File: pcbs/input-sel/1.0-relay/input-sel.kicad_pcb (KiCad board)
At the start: 2 copper layers, 85 x 55 mm, 54 parts, among them J1 Conn_01x03_Pin, J10 Conn_01x04_Pin, J2 Conn_01x03_Pin, J3 Conn_01x03_Pin, J4 Conn_01x03_Pin, J5 Conn_01x03_Pin, J6 Conn_01x03_Pin, J7 Conn_01x02_Pin, J8 Conn_01x02_Pin, J9 Conn_01x03_Pin, K1 EC2-5NU, K2 EC2-5NU, K3 EC2-5NU, K4 EC2-5NU, K5 EC2-5NU, K6 EC2-5NU, U1 CD74AC238, U2 TCMT4600, U3 TCMT4600

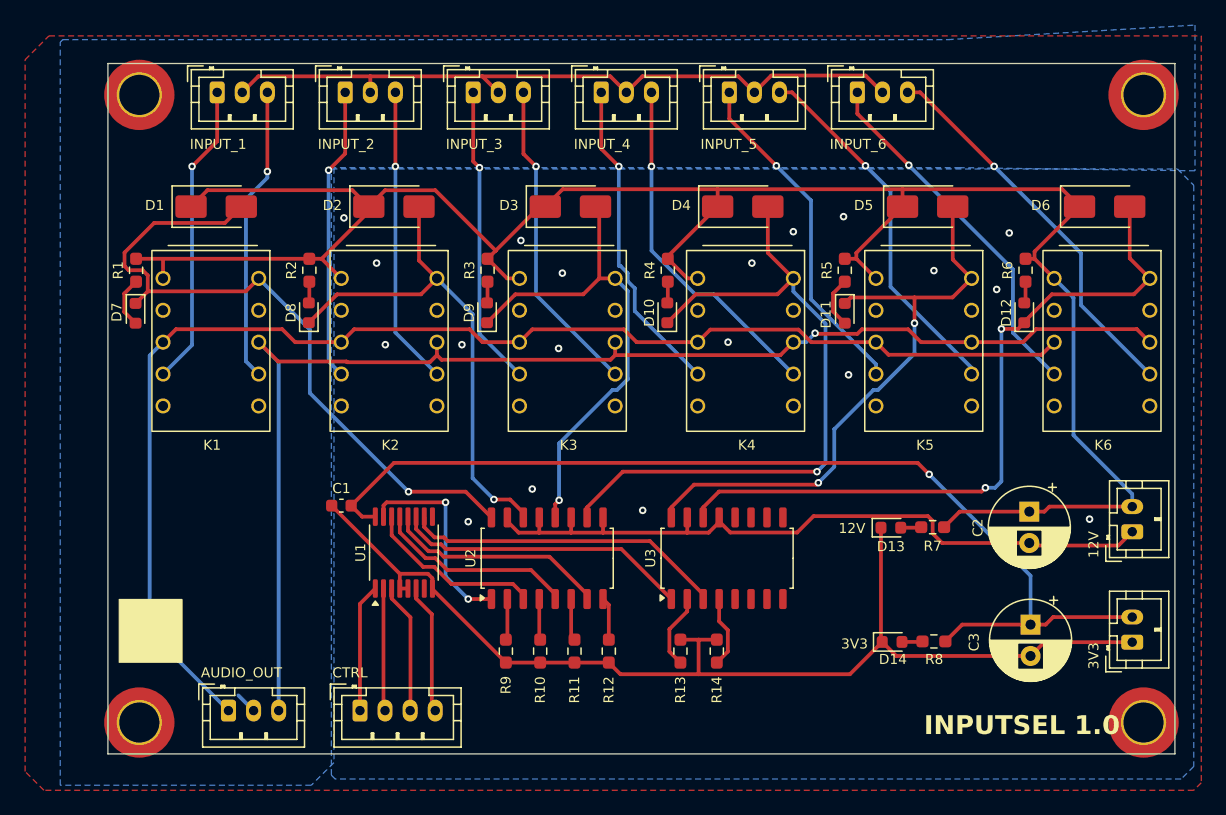
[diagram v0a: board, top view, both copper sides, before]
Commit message: Updates to pcbs
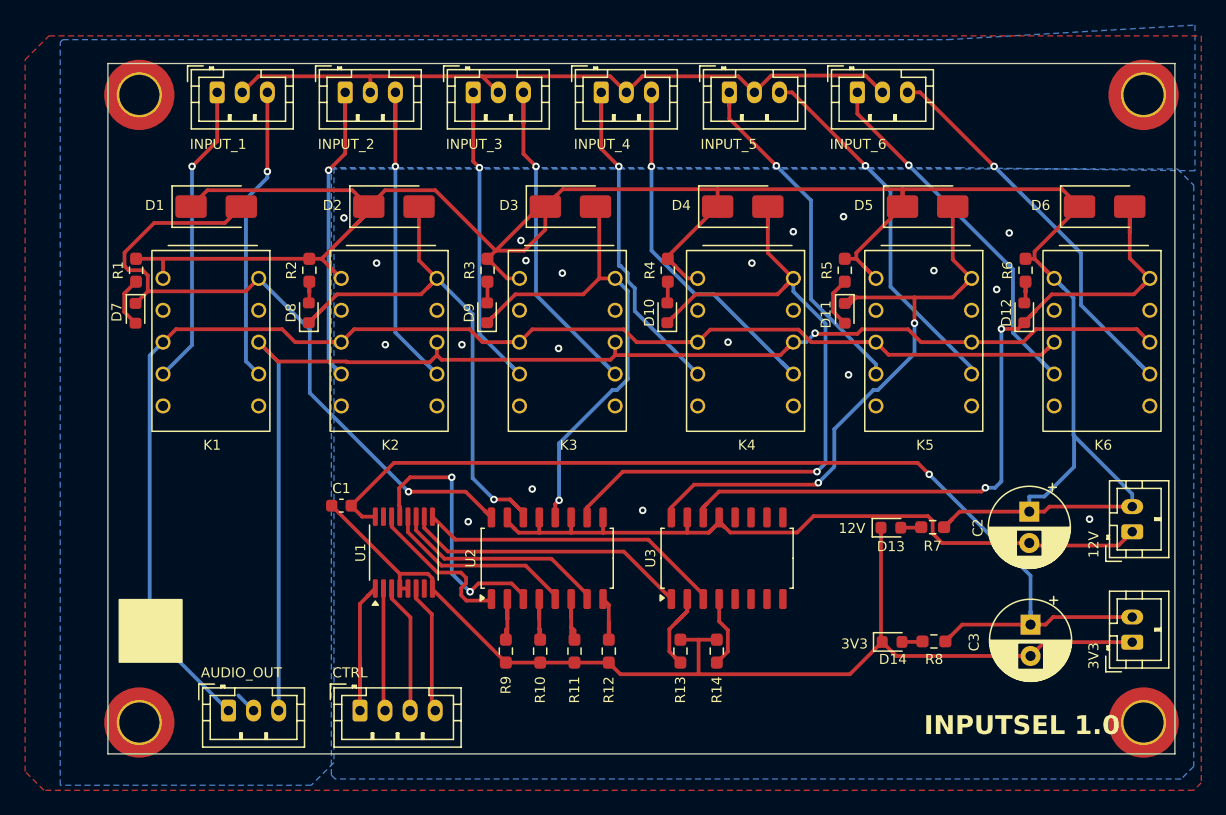
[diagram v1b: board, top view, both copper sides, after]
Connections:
- U1 pad 10: RELAY6 -> RELAY5
- U1 pad 11: RELAY5 -> RELAY4
- U1 pad 12: RELAY4 -> RELAY3
- U1 pad 13: RELAY3 -> RELAY2
- U1 pad 14: RELAY2 -> RELAY1
- U1 pad 15: RELAY1 -> unconnected-(U1-Y0-Pad15)
- U1 pad 9: unconnected-(U1-Y6-Pad9) -> RELAY6
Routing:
- net 12V: track 169.2 -> 198.7 mm
- net RELAY2: track 13.9 -> 21.8 mm, vias 0 -> 2
- net Net-(D12-K): track 57.4 -> 62.8 mm
- net CTRL1: track 10.2 -> 15.3 mm
- net RELAY_GND: track 58.0 -> 62.9 mm
- net Net-(D2-A): track 40.3 -> 45.1 mm
- net OUT_L: track 107.6 -> 112.1 mm
- net RCA2_R: track 23.8 -> 28.0 mm
- net RCA4_R: track 28.0 -> 32.2 mm
- net Net-(D10-K): track 55.1 -> 59.3 mm
- net RCA3_L: track 24.0 -> 28.0 mm
- net RCA3_R: track 25.5 -> 29.2 mm
- net RELAY1: track 16.2 -> 12.6 mm, vias 2 -> 0
- net RCA2_L: track 23.4 -> 26.6 mm
- net Net-(R13-Pad1): track 6.02 -> 8.89 mm
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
